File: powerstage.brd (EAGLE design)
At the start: 42 x 43.5 mm, 42 parts, among them CON1 PINHEAD_1X10-2-FEMALE, CON2 BATTERY_CON-2P-XT30-RA, CON3 PINHEAD_1X10-2-FEMALE, IC5 MCP9700, Q1 BUK9K6R2-40E,115, Q2 BUK9K6R2-40E,115, Q3 BUK9K6R2-40E,115

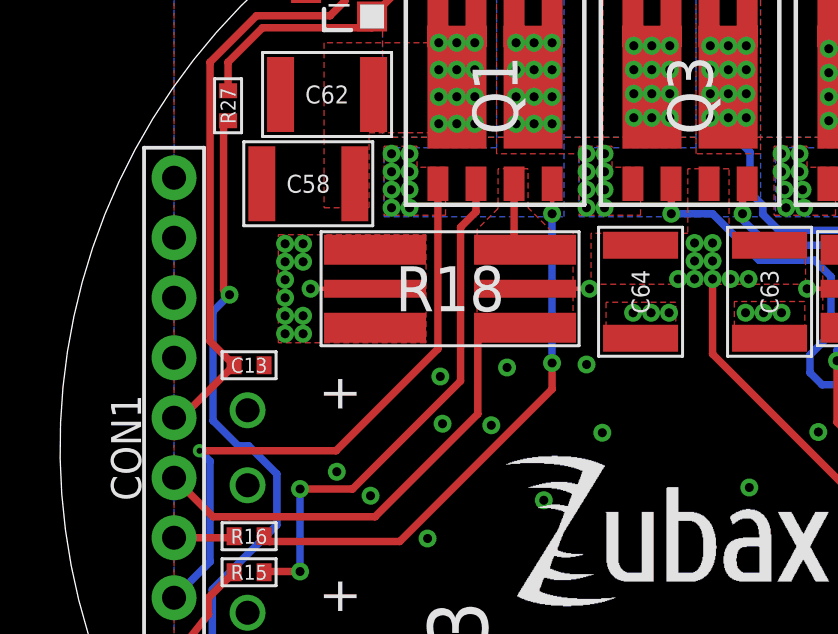
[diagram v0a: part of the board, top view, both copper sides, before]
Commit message: inner layers update
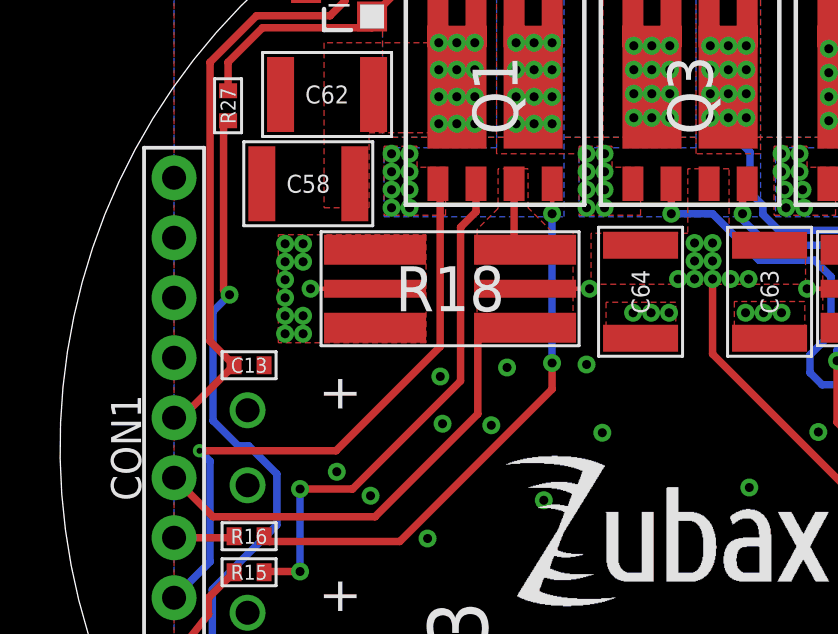
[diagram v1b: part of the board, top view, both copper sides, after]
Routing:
- net PHASE_A_CURRENT_SHUNT_N: track 36.9 -> 36.3 mm
- net PHASE_B_CURRENT_SHUNT_P: track 18.0 -> 17.4 mm
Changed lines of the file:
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@@
 <layer number="14" name="Route14" color="22" fill="1" visible="no" active="no"/>
 <layer number="15" name="Route15" color="46" fill="6" visible="no" active="yes"/>
-<layer number="16" name="Bottom" color="1" fill="1" visible="yes" active="yes"/>
+<layer number="16" name="Bottom" color="1" fill="1" visible="no" active="yes"/>
 <layer number="17" name="Pads" color="2" fill="1" visible="yes" active="yes"/>
 <layer number="18" name="Vias" color="2" fill="1" visible="yes" active="yes"/>
@@
 <layer number="20" name="Dimension" color="24" fill="1" visible="yes" active="yes"/>
 <layer number="21" name="tPlace" color="7" fill="1" visible="no" active="yes"/>
-<layer number="22" name="bPlace" color="7" fill="1" visible="yes" active="yes"/>
+<layer number="22" name="bPlace" color="7" fill="1" visible="no" active="yes"/>
 <layer number="23" name="tOrigins" color="15" fill="1" visible="no" active="yes"/>
-<layer number="24" name="bOrigins" color="15" fill="1" visible="yes" active="yes"/>
+<layer number="24" name="bOrigins" color="15" fill="1" visible="no" active="yes"/>
 <layer number="25" name="tNames" color="7" fill="1" visible="no" active="yes"/>
-<layer number="26" name="bNames" color="7" fill="1" visible="yes" active="yes"/>
+<layer number="26" name="bNames" color="7" fill="1" visible="no" active="yes"/>
 <layer number="27" name="tValues" color="7" fill="1" visible="no" active="yes"/>
 <layer number="28" name="bValues" color="7" fill="1" visible="no" active="yes"/>
@@
 <layer number="50" name="dxf" color="7" fill="1" visible="no" active="yes"/>
 <layer number="51" name="tDocu" color="7" fill="1" visible="no" active="yes"/>
-<layer number="52" name="bDocu" color="7" fill="1" visible="yes" active="yes"/>
+<layer number="52" name="bDocu" color="7" fill="1" visible="no" active="yes"/>
 <layer number="53" name="tGND_GNDA" color="7" fill="9" visible="no" active="no"/>
 <layer number="54" name="bGND_GNDA" color="1" fill="9" visible="no" active="no"/>
@@
 </layers>
 <board>
-<fusionsync huburn="a.cGVyc29uYWw6dWUyYWE4ZDY4" projecturn="a.cGVyc29uYWw6dWUyYWE4ZDY4IzIwMTgxMTA4MTU5MTUwNTA2" f3durn="urn:adsk.wipprod:dm.lineage:PNkJALQsRiGXmceaXmEg1A" pcbguid="a30d68d2-795d-4aa0-9250-ee42eeb516a6" lastpulledtime="" lastsyncedchangeguid="d8c6bf63-8608-d522-5299-755ff265eaea"/>
+<fusionsync huburn="a.cGVyc29uYWw6dWUyYWE4ZDY4" projecturn="a.cGVyc29uYWw6dWUyYWE4ZDY4IzIwMTgxMTA4MTU5MTUwNTA2" f3durn="urn:adsk.wipprod:dm.lineage:PNkJALQsRiGXmceaXmEg1A" pcbguid="a30d68d2-795d-4aa0-9250-ee42eeb516a6" lastpulledtime="" lastsyncedchangeguid="5c4f4f1c-28fc-b0fa-ed4d-baeeaa0fb5fd"/>
 <plain>
 <wire x1="0" y1="0" x2="0" y2="21" width="0.1524" layer="49" style="shortdash" locked="yes"/>
@@
 </autorouter>
 <elements>
-<element name="A" library="PADS" library_urn="urn:adsk.eagle:library:3188696" package="HOLE_2" package3d_urn="urn:adsk.eagle:package:4854323/1" value="PAD-HOLE_2" x="5" y="18" smashed="yes">
+<element name="A" library="PADS" library_urn="urn:adsk.eagle:library:3188696" package="HOLE_2" package3d_urn="urn:adsk.eagle:package:4854323/1" value="PAD-HOLE_2" x="5" y="18" locked="yes" smashed="yes">
 <attribute name="BOM" value="EXCLUDE" x="5" y="18" size="1.778" layer="27" display="off"/>
 <attribute name="NAME" x="5" y="20" size="1" layer="25" font="vector" ratio="15" align="center"/>
@@
 <attribute name="VALUE" x="14.7" y="1.75" size="0.5" layer="27" font="vector" ratio="15" rot="R180" align="center"/>
 </element>
-<element name="B" library="PADS" library_urn="urn:adsk.eagle:library:3188696" package="HOLE_2" package3d_urn="urn:adsk.eagle:package:4854323/1" value="PAD-HOLE_2" x="-5" y="18" smashed="yes">
+<element name="B" library="PADS" library_urn="urn:adsk.eagle:library:3188696" package="HOLE_2" package3d_urn="urn:adsk.eagle:package:4854323/1" value="PAD-HOLE_2" x="-5" y="18" locked="yes" smashed="yes">
 <attribute name="BOM" value="EXCLUDE" x="-5" y="18" size="1.778" layer="27" display="off"/>
 <attribute name="NAME" x="-5" y="20" size="1" layer="25" font="vector" ratio="15" align="center"/>
@@
 <attribute name="VALUE" x="-14.7" y="-2.05" size="0.5" layer="27" font="vector" ratio="15" align="center"/>
 </element>
-<element name="C" library="PADS" library_urn="urn:adsk.eagle:library:3188696" package="HOLE_2" package3d_urn="urn:adsk.eagle:package:4854323/1" value="PAD-HOLE_2" x="0" y="18" smashed="yes">
+<element name="C" library="PADS" library_urn="urn:adsk.eagle:library:3188696" package="HOLE_2" package3d_urn="urn:adsk.eagle:package:4854323/1" value="PAD-HOLE_2" x="0" y="18" locked="yes" smashed="yes">
 <attribute name="BOM" value="EXCLUDE" x="0" y="18" size="1.778" layer="27" display="off"/>
 <attribute name="NAME" x="0" y="20" size="1" layer="25" font="vector" ratio="15" align="center"/>
@@
 <vertex x="11.125" y="8.825"/>
 </polygon>
-<polygon width="0.3" layer="2">
+<polygon width="0.2" layer="2">
 <vertex x="-17.2" y="19.4"/>
 <vertex x="-17.2" y="-20"/>
@@
 <contactref element="Q2" pad="1"/>
 <wire x1="4.595" y1="8.8" x2="4.595" y2="9.2" width="0.1524" layer="1"/>
-<polygon width="0.1524" layer="1" thermals="no">
+<polygon width="0.2" layer="1" thermals="no">
 <vertex x="6.7" y="9.8"/>
 <vertex x="6.7" y="15.7"/>
@@
 <wire x1="7.2128625" y1="1.65" x2="8.4" y2="2.8371375" width="0.15" layer="15"/>
 <contactref element="CON1" pad="8"/>
-<wire x1="-16.6" y1="4.05" x2="-17.5" y2="4.95" width="0.15" layer="15"/>
-<wire x1="-17.5" y1="4.95" x2="-17.2" y2="5" width="0.15" layer="15"/>
+<wire x1="-16.25" y1="4.05" x2="-17.2" y2="5" width="0.15" layer="15"/>
 <wire x1="7.2128625" y1="1.65" x2="-12.7378625" y2="1.65" width="0.15" layer="15"/>
 <wire x1="-12.7378625" y1="1.65" x2="-15.1378625" y2="4.05" width="0.15" layer="15"/>
-<wire x1="-15.1378625" y1="4.05" x2="-16.6" y2="4.05" width="0.15" layer="15"/>
+<wire x1="-15.1378625" y1="4.05" x2="-16.25" y2="4.05" width="0.15" layer="15"/>
 </signal>
 <signal name="PHASE_A_CURRENT_SHUNT_P">
@@
 <wire x1="-15.30606875" y1="3.74393125" x2="-12.9121375" y2="1.35" width="0.15" layer="15"/>
 <contactref element="CON1" pad="7"/>
-<wire x1="-15.30606875" y1="3.74393125" x2="-16.60606875" y2="3.74393125" width="0.15" layer="15"/>
-<wire x1="-16.60606875" y1="3.74393125" x2="-17.35" y2="3" width="0.15" layer="15"/>
-<wire x1="-17.2" y1="3" x2="-17.35" y2="3" width="0.15" layer="15"/>
+<wire x1="-15.30606875" y1="3.74393125" x2="-16.28106875" y2="3.74393125" width="0.15" layer="15"/>
+<wire x1="-16.28106875" y1="3.74393125" x2="-17.025" y2="3" width="0.15" layer="15"/>
+<wire x1="-17.025" y1="3" x2="-17.2" y2="3" width="0.15" layer="15"/>
 <wire x1="-12.9121375" y1="1.35" x2="7.3871375" y2="1.35" width="0.15" layer="15"/>
 </signal>
@@
 <wire x1="-10.7378625" y1="6.65" x2="-12.2878625" y2="8.2" width="0.15" layer="15"/>
 <wire x1="-10.7378625" y1="6.65" x2="-8.4378625" y2="6.65" width="0.15" layer="15"/>
-<wire x1="-16.7" y1="8.2" x2="-17.2" y2="9" width="0.15" layer="15"/>
-<wire x1="-12.2878625" y1="8.2" x2="-16.7" y2="8.2" width="0.15" layer="15"/>
+<wire x1="-16.4" y1="8.2" x2="-17.2" y2="9" width="0.15" layer="15"/>
+<wire x1="-12.2878625" y1="8.2" x2="-16.4" y2="8.2" width="0.15" layer="15"/>
 </signal>
 <signal name="PHASE_B_CURRENT_SHUNT_P">
@@
 <wire x1="-8.15" y1="5.55" x2="-8.15" y2="5.9378625" width="0.15" layer="15"/>
 <wire x1="-8.5621375" y1="6.35" x2="-8.15" y2="5.9378625" width="0.15" layer="15"/>
-<wire x1="-16.7" y1="7.9" x2="-17.5" y2="7.1" width="0.15" layer="15"/>
-<wire x1="-17.5" y1="7.1" x2="-17.2" y2="7" width="0.15" layer="15"/>
-<wire x1="-16.7" y1="7.9" x2="-12.4121375" y2="7.9" width="0.15" layer="15"/>
+<wire x1="-16.4" y1="7.9" x2="-17.2" y2="7.1" width="0.15" layer="15"/>
+<wire x1="-17.2" y1="7.1" x2="-17.2" y2="7" width="0.15" layer="15"/>
+<wire x1="-16.4" y1="7.9" x2="-12.4121375" y2="7.9" width="0.15" layer="15"/>
 <wire x1="-12.4121375" y1="7.9" x2="-10.8621375" y2="6.35" width="0.15" layer="15"/>
 <wire x1="-10.8621375" y1="6.35" x2="-8.5621375" y2="6.35" width="0.15" layer="15"/>
@@
 <contactref element="Q3" pad="5" route="any" routetag="T2.D"/>
 <contactref element="Q3" pad="1"/>
-<polygon width="0.1524" layer="1" thermals="no" rank="3">
+<polygon width="0.2" layer="1" thermals="no" rank="3">
 <vertex x="0.2" y="9.8"/>
 <vertex x="0.2" y="15.8"/>
@@
 <contactref element="Q1" pad="1"/>
 <contactref element="B" pad="P$1"/>
-<polygon width="0.1524" layer="1" thermals="no" rank="2">
+<polygon width="0.2" layer="1" thermals="no" rank="2">
 <vertex x="-6.45" y="9.8"/>
 <vertex x="-6.45" y="19.4"/>
@@
 <vertex x="-2.9" y="9.8"/>
 </polygon>
-<wire x1="-8.405" y1="8.8" x2="-8.405" y2="3.295" width="0.25" layer="1"/>
-<wire x1="-8.405" y1="3.295" x2="-11.8" y2="-0.1" width="0.25" layer="1"/>
+<wire x1="-8.405" y1="8.8" x2="-8.33" y2="8.725" width="0.25" layer="1"/>
+<wire x1="-8.33" y1="8.725" x2="-8.33" y2="3.37" width="0.25" layer="1"/>
+<wire x1="-8.33" y1="3.37" x2="-11.8" y2="-0.1" width="0.25" layer="1"/>
 <polygon width="0.1524" layer="1" thermals="no">
 <vertex x="-8.15" y="9.35"/>

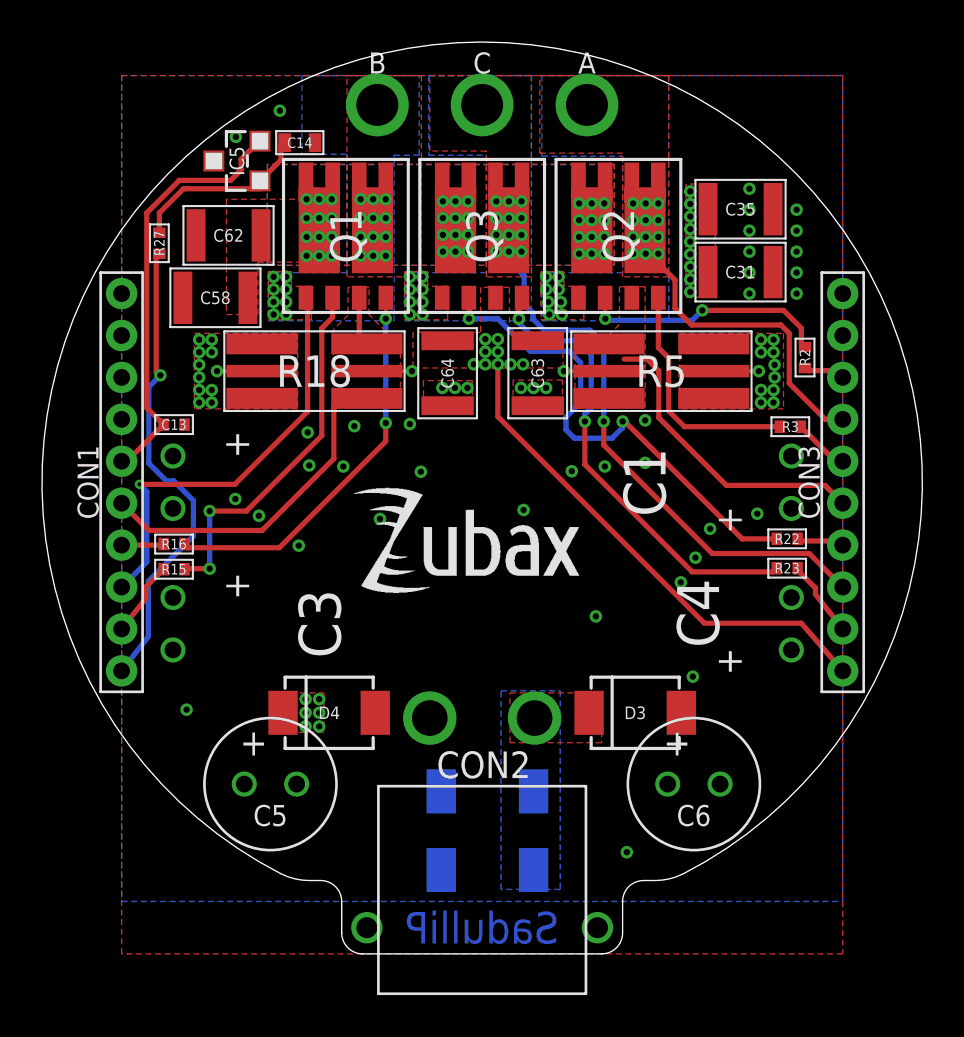
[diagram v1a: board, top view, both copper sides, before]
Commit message: poly update
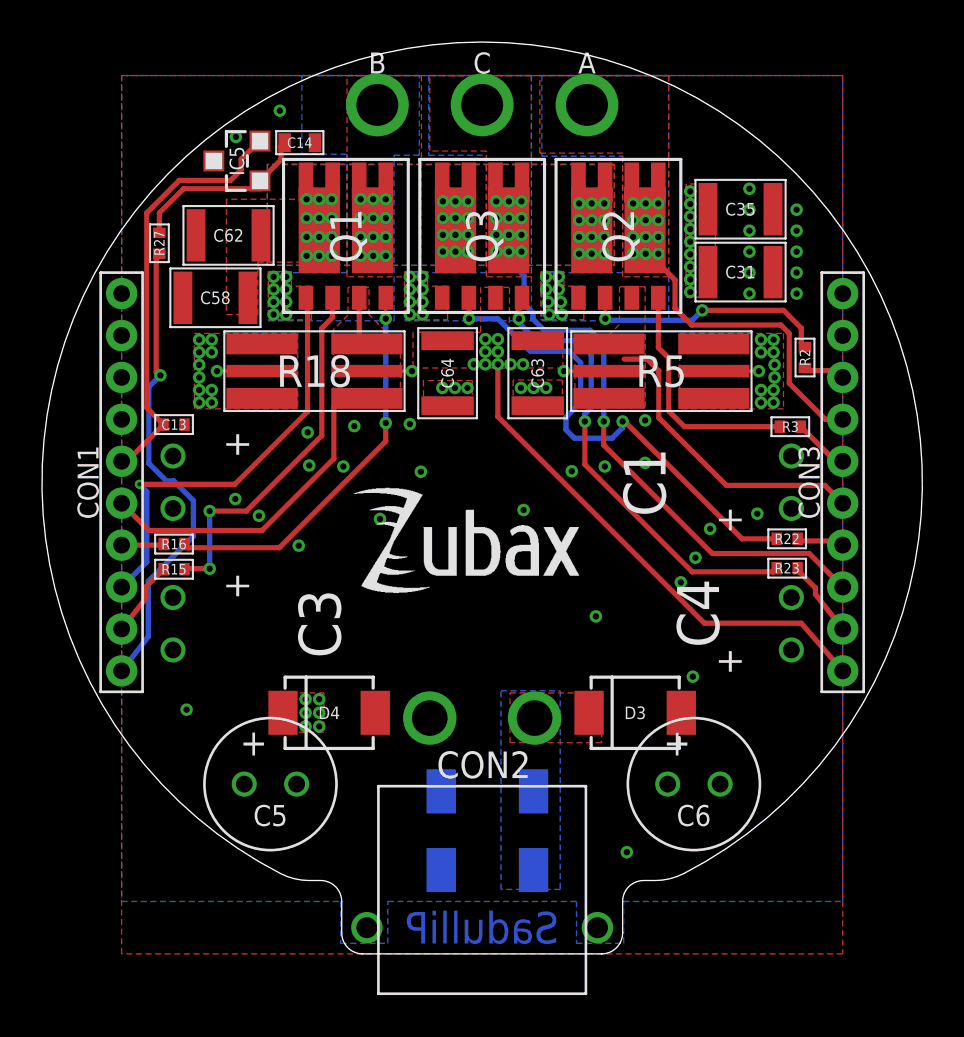
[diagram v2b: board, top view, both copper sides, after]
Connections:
- net PGND: now also CON2.P$3, CON2.P$4
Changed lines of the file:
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@@
 <drawing>
 <settings>
-<setting alwaysvectorfont="yes"/>
+<setting alwaysvectorfont="no"/>
 <setting verticaltext="up"/>
 </settings>
-<grid distance="0.025" unitdist="mm" unit="mm" style="lines" multiple="1" display="no" altdistance="5" altunitdist="mil" altunit="mil"/>
+<grid distance="0.25" unitdist="mm" unit="mm" style="lines" multiple="1" display="yes" altdistance="5" altunitdist="mil" altunit="mil"/>
 <layers>
 <layer number="1" name="Top" color="4" fill="1" visible="no" active="yes"/>
-<layer number="2" name="Route2" color="43" fill="3" visible="yes" active="yes"/>
+<layer number="2" name="Route2" color="43" fill="3" visible="no" active="yes"/>
 <layer number="3" name="Route3" color="17" fill="1" visible="no" active="no"/>
 <layer number="4" name="Route4" color="18" fill="1" visible="no" active="no"/>
@@
 <layer number="14" name="Route14" color="22" fill="1" visible="no" active="no"/>
 <layer number="15" name="Route15" color="46" fill="6" visible="no" active="yes"/>
-<layer number="16" name="Bottom" color="1" fill="1" visible="no" active="yes"/>
+<layer number="16" name="Bottom" color="1" fill="1" visible="yes" active="yes"/>
 <layer number="17" name="Pads" color="2" fill="1" visible="yes" active="yes"/>
 <layer number="18" name="Vias" color="2" fill="1" visible="yes" active="yes"/>
@@
 <layer number="20" name="Dimension" color="24" fill="1" visible="yes" active="yes"/>
 <layer number="21" name="tPlace" color="7" fill="1" visible="no" active="yes"/>
-<layer number="22" name="bPlace" color="7" fill="1" visible="no" active="yes"/>
+<layer number="22" name="bPlace" color="7" fill="1" visible="yes" active="yes"/>
 <layer number="23" name="tOrigins" color="15" fill="1" visible="no" active="yes"/>
-<layer number="24" name="bOrigins" color="15" fill="1" visible="no" active="yes"/>
+<layer number="24" name="bOrigins" color="15" fill="1" visible="yes" active="yes"/>
 <layer number="25" name="tNames" color="7" fill="1" visible="no" active="yes"/>
-<layer number="26" name="bNames" color="7" fill="1" visible="no" active="yes"/>
-<layer number="27" name="tValues" color="7" fill="1" visible="no" active="yes"/>
+<layer number="26" name="bNames" color="7" fill="1" visible="yes" active="yes"/>
+<layer number="27" name="tValues" color="7" fill="1" visible="yes" active="yes"/>
 <layer number="28" name="bValues" color="7" fill="1" visible="no" active="yes"/>
 <layer number="29" name="tStop" color="7" fill="3" visible="no" active="yes"/>
@@
 <layer number="50" name="dxf" color="7" fill="1" visible="no" active="yes"/>
 <layer number="51" name="tDocu" color="7" fill="1" visible="no" active="yes"/>
-<layer number="52" name="bDocu" color="7" fill="1" visible="no" active="yes"/>
+<layer number="52" name="bDocu" color="7" fill="1" visible="yes" active="yes"/>
 <layer number="53" name="tGND_GNDA" color="7" fill="9" visible="no" active="no"/>
 <layer number="54" name="bGND_GNDA" color="1" fill="9" visible="no" active="no"/>
@@
 <contactref element="CON2" pad="-"/>
 <polygon width="0.1524" layer="16" rank="5">
-<vertex x="0" y="19.4"/>
+<vertex x="17.2" y="19.4"/>
 <vertex x="-17.2" y="19.4"/>
 <vertex x="-17.2" y="-20"/>
+<vertex x="-6.75" y="-20"/>
+<vertex x="-6.75" y="-22"/>
+<vertex x="-4.5" y="-22"/>
+<vertex x="-4.5" y="-20"/>
+<vertex x="4.5" y="-20"/>
+<vertex x="4.5" y="-22"/>
+<vertex x="6.75" y="-22"/>
+<vertex x="6.75" y="-20"/>
 <vertex x="17.2" y="-20"/>
-<vertex x="17.2" y="19.4"/>
 </polygon>
 <via x="13.3" y="6.8" extent="1-16" drill="0.3" diameter="0.6"/>
@@
 <contactref element="D3" pad="A"/>
 <contactref element="D4" pad="A"/>
+<contactref element="CON2" pad="P$3"/>
+<contactref element="CON2" pad="P$4"/>
 </signal>
 <signal name="N$3">
